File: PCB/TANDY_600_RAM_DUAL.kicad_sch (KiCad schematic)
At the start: 8 parts, among them CN1 TANDY_600_RAM_BUS_plain_pins, CN2 TANDY_600_RAM_BUS_plain_pins, U1 AS6C2008A, U2 HC148, U3 1G02

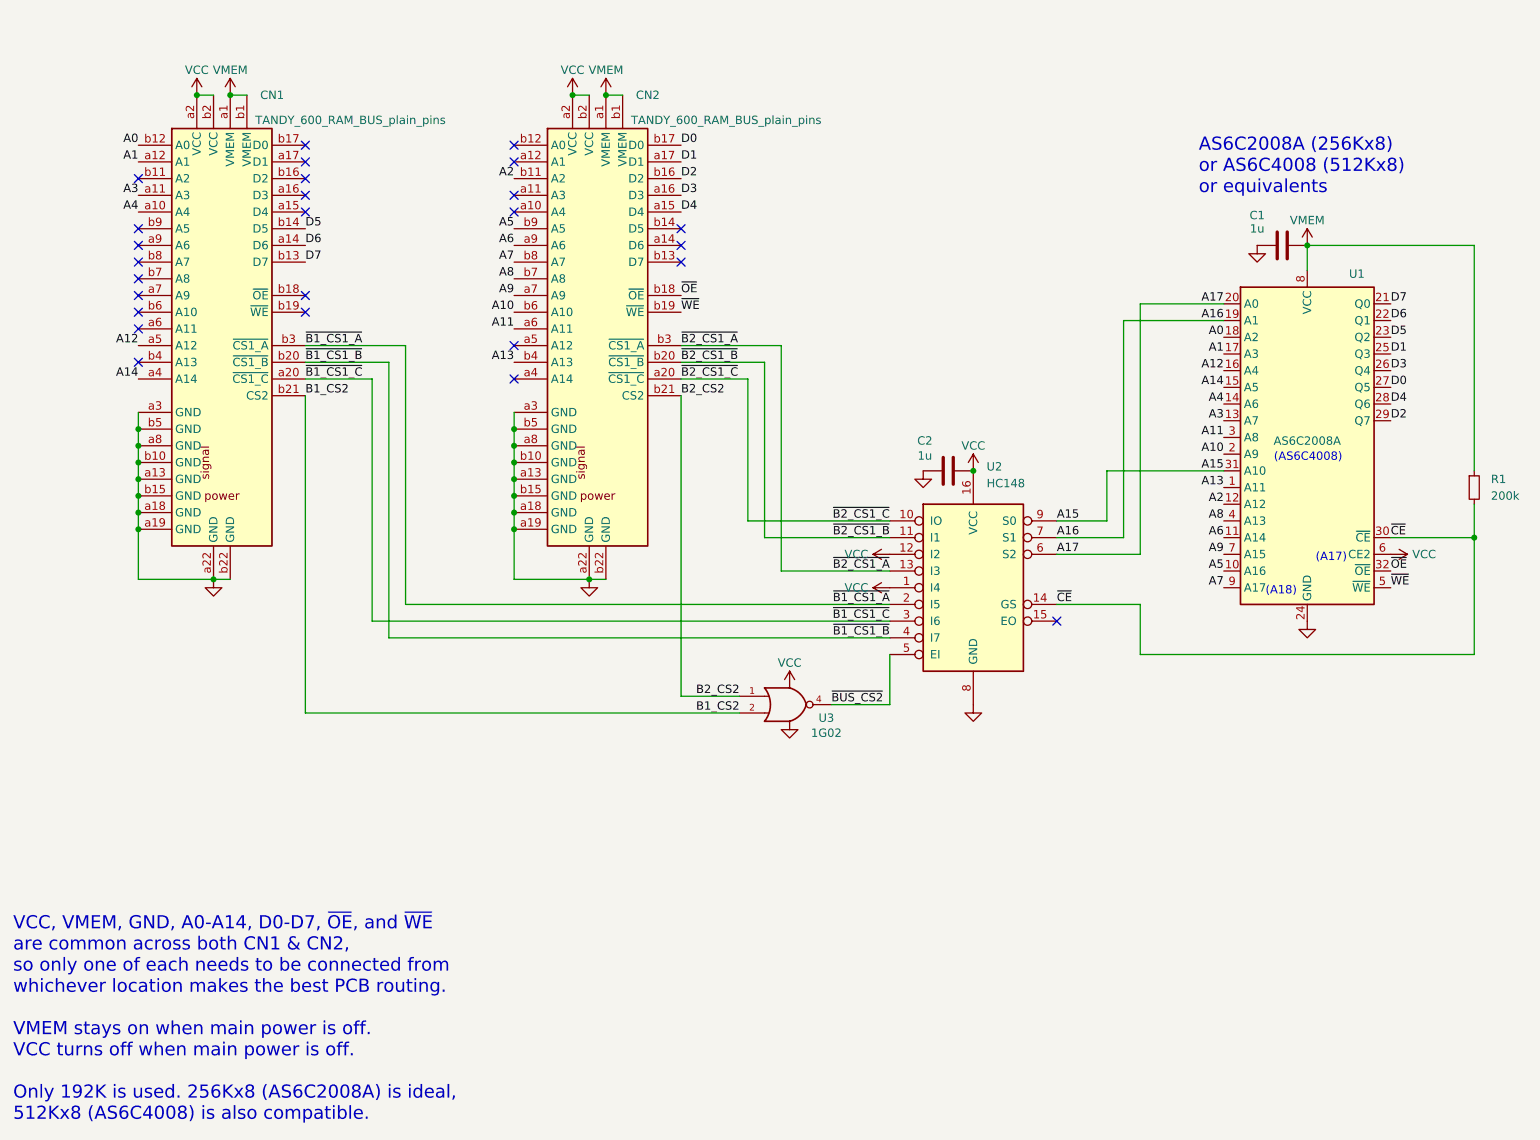
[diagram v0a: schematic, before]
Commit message: datasheets OPRM pinout
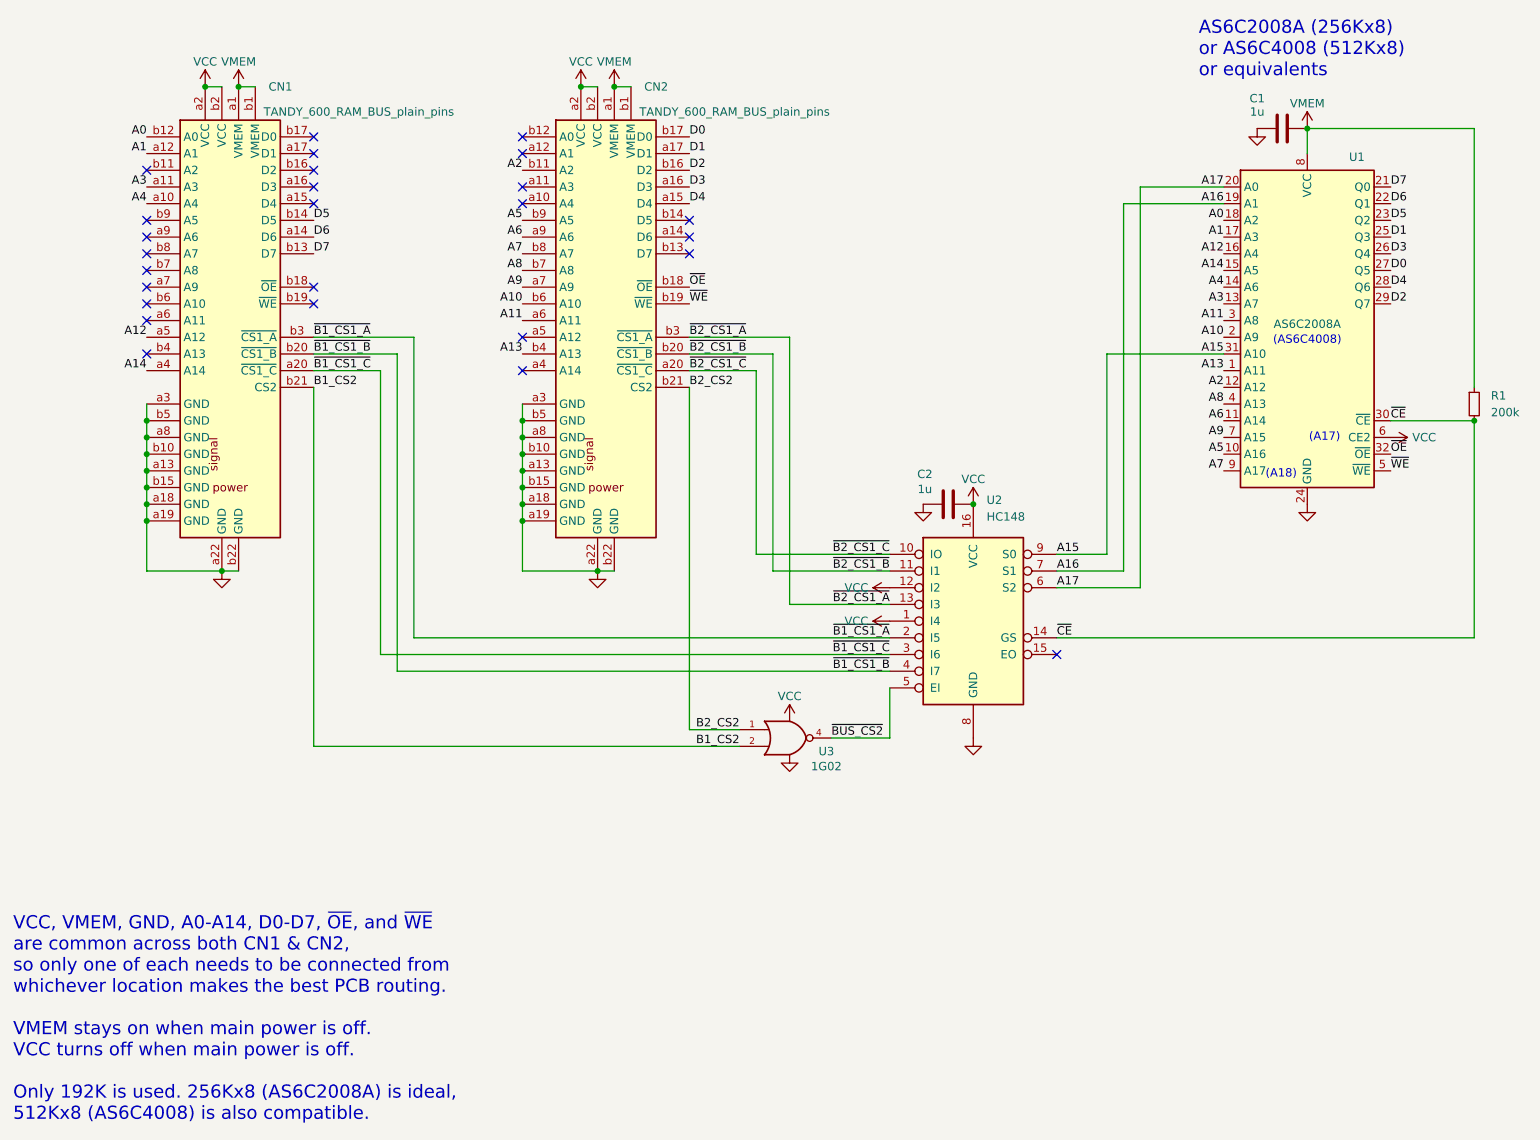
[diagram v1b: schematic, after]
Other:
- moved on the sheet: C1, C2, CN1, CN2, R1, U1, U2, U3
